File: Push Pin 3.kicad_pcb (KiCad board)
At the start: 2 copper layers, 95 x 77.4 mm, 43 parts, among them J1 Screw_Terminal_01x02, J10 Screw_Terminal_01x02, J11 Screw_Terminal_01x02, J12 Screw_Terminal_01x02, J13 Screw_Terminal_01x02, J2 Screw_Terminal_01x02, J3 Screw_Terminal_01x02, J4 Screw_Terminal_01x02, J5 Screw_Terminal_01x02, J6 Screw_Terminal_01x02, J7 Screw_Terminal_01x02, J8 Screw_Terminal_01x02, J9 Screw_Terminal_01x02, SW1 SW_DPDT_x2, SW2 SW_DPDT_x2, SW3 SW_DPDT_x2, U1 LM2596S-ADJ

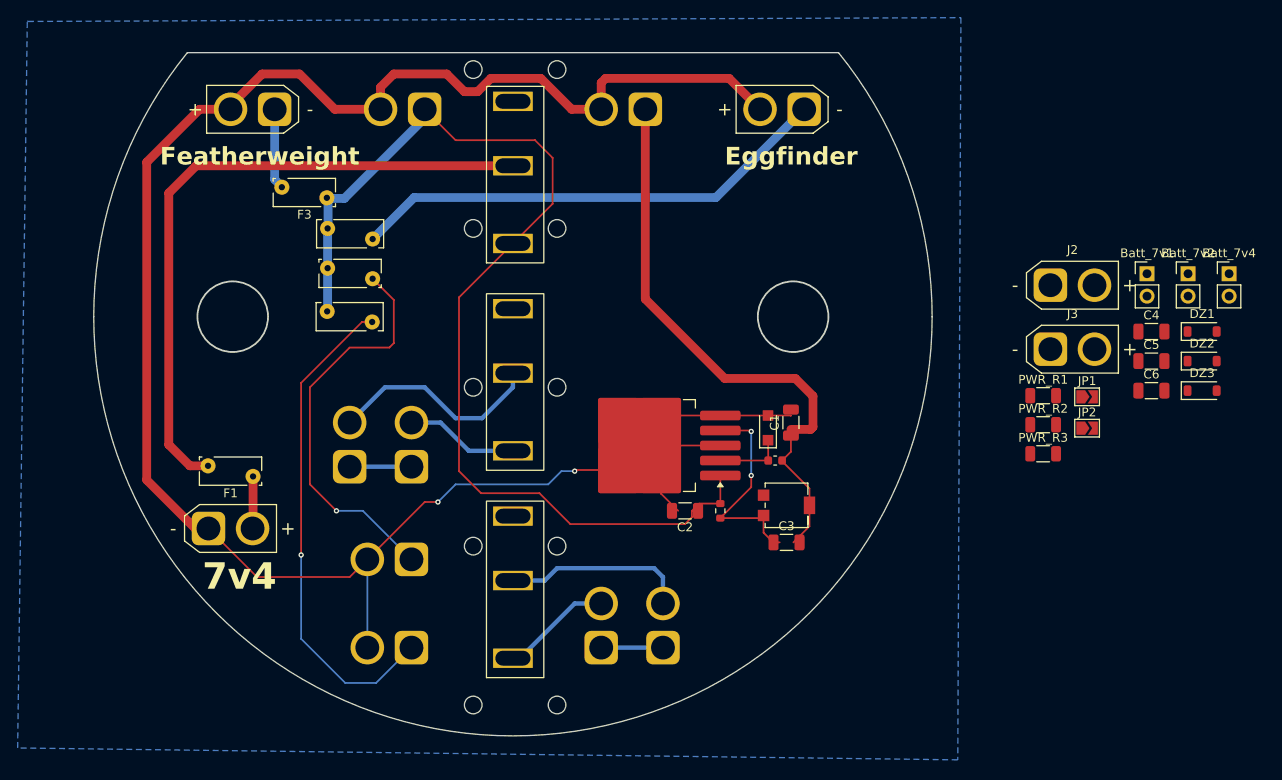
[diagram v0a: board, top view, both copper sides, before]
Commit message: PCB au complet
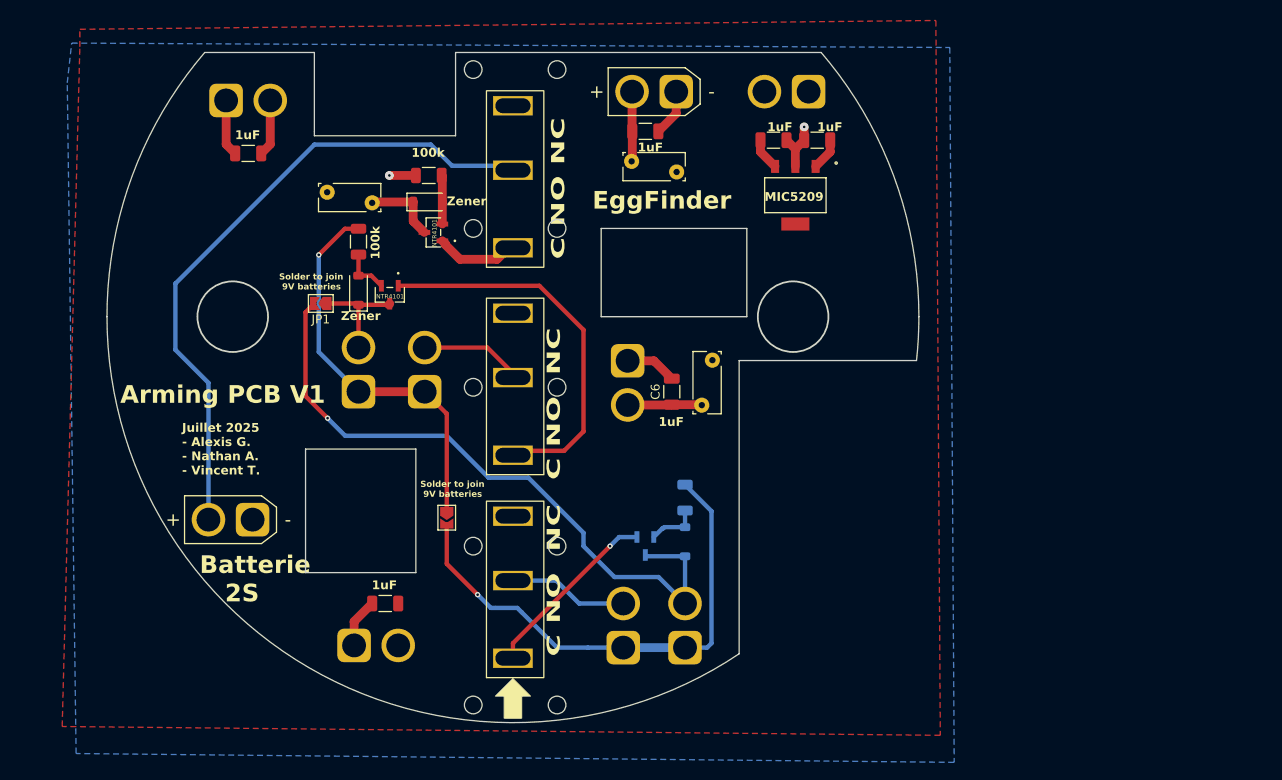
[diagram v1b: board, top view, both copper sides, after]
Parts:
- removed D2: D_Schottky, Diode_SMD:Nexperia_CFP3_SOD-123W
- removed F4, F5: Fuse, Fuse:Fuse_Bourns_MF-RHT050
- removed J10, J11, J12, J13, J8, J9: Screw_Terminal_01x02, Connector_AMASS:AMASS_XT30U-M_1x02_P5.0mm_Vertical
- removed L1: 47uH, Inductor_SMD:L_0603_1608Metric
- removed R1: 1k, Resistor_SMD:R_0603_1608Metric
- removed R2: 2k, Potentiometer_SMD:Potentiometer_Bourns_3214G_Horizontal
- removed SW1, SW2, SW3: SW_DPDT_x2, Library:Omrun_SS-01GL13
- removed U1: LM2596S-ADJ, Package_TO_SOT_SMD:TO-263-5_TabPin3
- added Q1: NTR4101PT1G, NTR4101PT1G:SOT-23-3_1P4X3P040_ONS, F.Cu at (141.0, 90.5)
- added Q2: NTR4101PT1G, NTR4101PT1G:SOT-23-3_1P4X3P040_ONS, B.Cu at (165.0, 126.0)
- added Q3: NTR4101PT1G, NTR4101PT1G:SOT-23-3_1P4X3P040_ONS, F.Cu at (136.0, 97.5)
- added SW4: SW_DPDT_x2, Library:Omrun_SS-01GL13, F.Cu at (150.0, 83.4)
- added SW5: SW_DPDT_x2, Library:Omrun_SS-01GL13, F.Cu at (150.0, 129.9)
- added SW6: SW_DPDT_x2, Library:Omrun_SS-01GL13, F.Cu at (150.0, 106.9)
- added U2: LDO_4v2-MIC5209-4.2YS-TR, footprints:SOT-223_S_MCH, F.Cu at (182.0, 86.2)
- Batt_7v1, Batt_7v2: footprint Connector_PinHeader_2.54mm:PinHeader_1x02_P2.54mm_Vertical -> Connector_AMASS:AMASS_XT30U-M_1x02_P5.0mm_Vertical; moved to B.Cu
- Batt_7v4: footprint Connector_PinHeader_2.54mm:PinHeader_1x02_P2.54mm_Vertical -> Connector_AMASS:AMASS_XT30U-M_1x02_P5.0mm_Vertical
- DZ2, J1, J2, J3, PWR_R2: moved to B.Cu
- J5: moved to F.Cu
- moved Batt_7v4 114.1 mm to (120.5, 123.0), turned to 180 degrees
- moved DZ3 96.3 mm to (132.5, 97.0), turned to 90 degrees
- moved DZ1 89.0 mm to (140.3, 87.0)
- moved Batt_7v2 87.5 mm to (140.0, 108.5), turned to 90 degrees
- moved JP1 87.5 mm to (128.2, 98.5), turned to 180 degrees
- moved PWR_R3 81.2 mm to (132.5, 91.5), turned to 90 degrees
- moved J6 79.3 mm to (117.5, 75.5), turned to 0 degrees
- moved J3 78.5 mm to (132.5, 108.5), turned to 90 degrees
- moved C3 75.3 mm to (120.0, 81.5), turned to 180 degrees
- moved PWR_R1 74.0 mm to (140.5, 84.0), turned to 180 degrees
- moved JP2 73.3 mm to (142.5, 122.8), turned to -90 degrees
- moved Batt_7v1 72.9 mm to (162.5, 137.5), turned to 90 degrees
- moved J7 67.2 mm to (183.5, 74.5), turned to 180 degrees
- moved DZ2 62.1 mm to (169.5, 125.5), turned to 90 degrees
- moved J2 58.3 mm to (169.5, 137.5), turned to 90 degrees
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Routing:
- net V-: track 223.8 -> 0.00 mm, vias 2 -> 0
- net V+: track 121.9 -> 0.00 mm
- net 9V: track 0.00 -> 74.4 mm, vias 0 -> 1
- net Net-(SW3A-B): track 74.2 -> 0.00 mm
- net Net-(Batt_7v4-Pin_2): track 0.00 -> 74.1 mm
- net Net-(J12-Pin_1): track 67.6 -> 0.00 mm
- net 9V_GND: track 0.00 -> 57.8 mm, vias 0 -> 1
- net Net-(J9-Pin_1): track 56.1 -> 0.00 mm, vias 1 -> 0
- net Net-(J10-Pin_1): track 55.0 -> 0.00 mm
- net Net-(J8-Pin_1): track 45.9 -> 0.00 mm
- net Net-(Batt_7v2-Pin_1): track 0.00 -> 45.2 mm, vias 0 -> 1
- net Net-(Q3-D): track 0.00 -> 44.3 mm
- net Net-(J4-Pin_2): track 25.8 -> 0.00 mm
- net Net-(U1-FB): track 24.6 -> 0.00 mm, vias 2 -> 0
- net GND: track 7.00 -> 31.5 mm, vias 0 -> 2
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- added copper zone on F.Cu, net 7v4
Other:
- board size 95 x 77.4 mm -> 92 x 75.9 mm
- board text added: "100k"
- board text added: "1uF"
- board text added: "9V"
- board text added: "Arming PCB V1"
- board text added: "Batterie 2S"
- board text added: "C NO NC"
- board text added: "Cameras"
- board text added: "Easymini"
- board text added: "EggFinder"
- board text added: "Juillet 2025 - Alexis G. - Nathan A. - Vincent T."
- board text added: "MIC5209"
- board text added: "NTR4101"
- board text added: "Solder to join 9V batteries"
- board text added: "Zener"
- board text removed: "7v4"
- board text removed: "Cam"
- board text removed: "EasyMini"
- board text removed: "Eggfinder"
- board text removed: "Featherweight"
